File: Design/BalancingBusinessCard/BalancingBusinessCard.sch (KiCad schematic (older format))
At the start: 8 parts

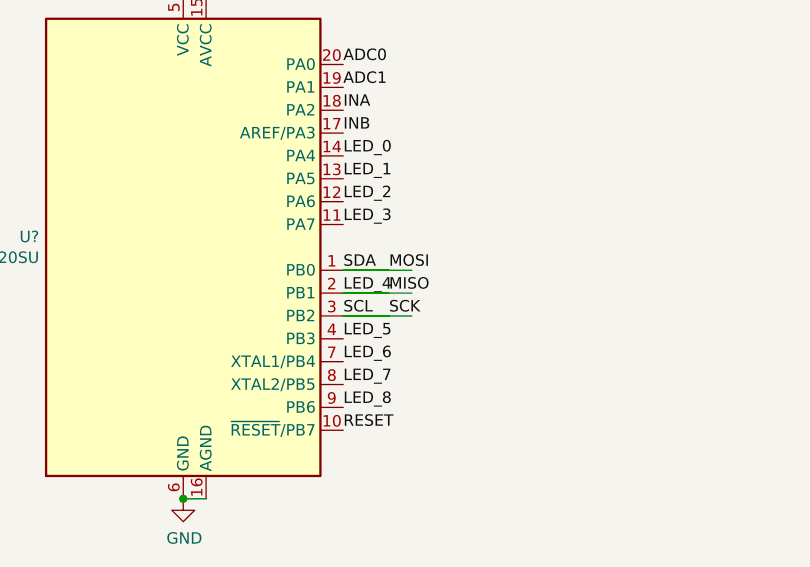
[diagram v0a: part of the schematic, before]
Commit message: Fixed stuff
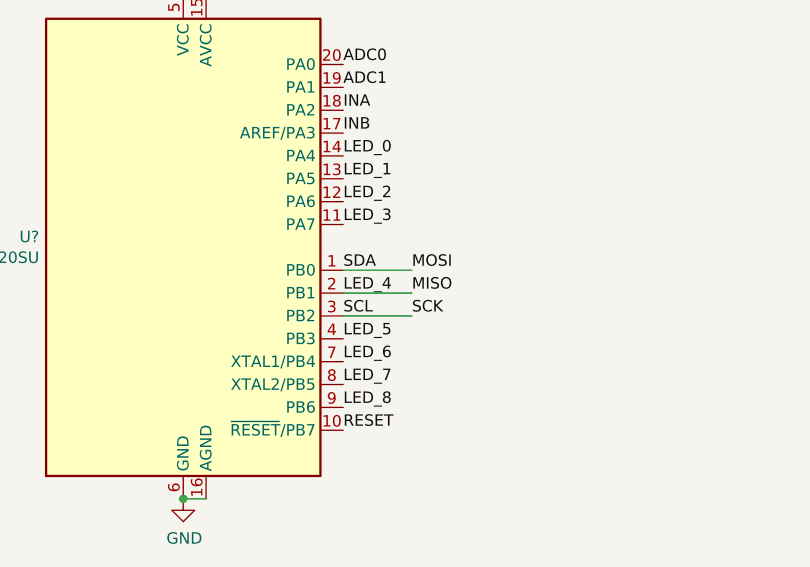
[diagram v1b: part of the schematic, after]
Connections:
- wire segments 20 -> 17
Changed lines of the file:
@@
 	1    0    0    -1
 $EndComp
-Text Label 4000 3850 0    50   ~ 0
+Text Label 4100 3850 0    50   ~ 0
 MOSI
-Wire Wire Line
-	4000 3850 3800 3850
-Text Label 4000 3950 0    50   ~ 0
+Text Label 4100 3950 0    50   ~ 0
 MISO
-Text Label 4000 4050 0    50   ~ 0
+Text Label 4100 4050 0    50   ~ 0
 SCK
-Wire Wire Line
-	4000 4050 3800 4050
-Wire Wire Line
-	4000 3950 3800 3950
 Text Label 7500 4200 2    50   ~ 0
 VCL
@@
 LED_8
 Wire Wire Line
-	3800 3850 4100 3850
-Wire Wire Line
-	4100 3950 3800 3950
-Wire Wire Line
-	3800 4050 4100 4050
-Wire Wire Line
 	3200 4850 3100 4850
 Connection ~ 3100 4850
@@
 	1    0    0    -1
 $EndComp
+Wire Wire Line
+	3800 3850 4100 3850
+Wire Wire Line
+	3800 4050 4100 4050
+Wire Wire Line
+	3800 3950 4100 3950
 $EndSCHEMATC
